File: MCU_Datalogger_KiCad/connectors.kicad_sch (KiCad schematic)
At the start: 4 parts, among them J1 Conn_01x04_Male, J2 Conn_01x04_Male, J3 Conn_01x09_Male, J4 Conn_02x03_Odd_Even

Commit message: Footprint association
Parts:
- J1: footprint (none) -> Connector_PinHeader_2.54mm:PinHeader_1x04_P2.54mm_Vertical
- J2: footprint (none) -> Connector_PinHeader_2.54mm:PinHeader_1x04_P2.54mm_Horizontal
- J3: footprint (none) -> Connector_PinHeader_2.54mm:PinHeader_1x09_P2.54mm_Vertical
- J4: footprint (none) -> Connector_PinHeader_2.54mm:PinHeader_2x03_P2.54mm_Vertical
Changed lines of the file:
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@@
     (property "Reference" "J2" (id 0) (at 65.405 30.48 0))
     (property "Value" "Conn_01x04_Male" (id 1) (at 65.405 33.02 0))
-    (property "Footprint" "" (id 2) (at 64.77 38.1 0)
+    (property "Footprint" "Connector_PinHeader_2.54mm:PinHeader_1x04_P2.54mm_Horizontal" (id 2) (at 64.77 38.1 0)
       (effects (font (size 1.27 1.27)) hide)
     )
@@
     (property "Reference" "J3" (id 0) (at 93.345 25.4 0))
     (property "Value" "Conn_01x09_Male" (id 1) (at 93.345 27.94 0))
-    (property "Footprint" "" (id 2) (at 92.71 40.64 0)
+    (property "Footprint" "Connector_PinHeader_2.54mm:PinHeader_1x09_P2.54mm_Vertical" (id 2) (at 92.71 40.64 0)
       (effects (font (size 1.27 1.27)) hide)
     )
@@
     (property "Reference" "J4" (id 0) (at 118.11 29.21 0))
     (property "Value" "Conn_02x03_Odd_Even" (id 1) (at 118.11 31.75 0))
-    (property "Footprint" "" (id 2) (at 116.84 38.1 0)
+    (property "Footprint" "Connector_PinHeader_2.54mm:PinHeader_2x03_P2.54mm_Vertical" (id 2) (at 116.84 38.1 0)
       (effects (font (size 1.27 1.27)) hide)
     )
@@
     (property "Reference" "J1" (id 0) (at 40.005 31.75 0))
     (property "Value" "Conn_01x04_Male" (id 1) (at 40.005 34.29 0))
-    (property "Footprint" "" (id 2) (at 39.37 39.37 0)
+    (property "Footprint" "Connector_PinHeader_2.54mm:PinHeader_1x04_P2.54mm_Vertical" (id 2) (at 39.37 39.37 0)
       (effects (font (size 1.27 1.27)) hide)
     )

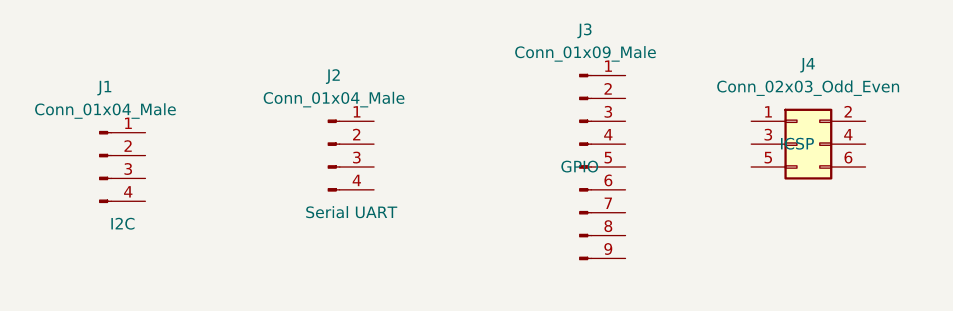
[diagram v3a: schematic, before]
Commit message: Wiring sheet 2
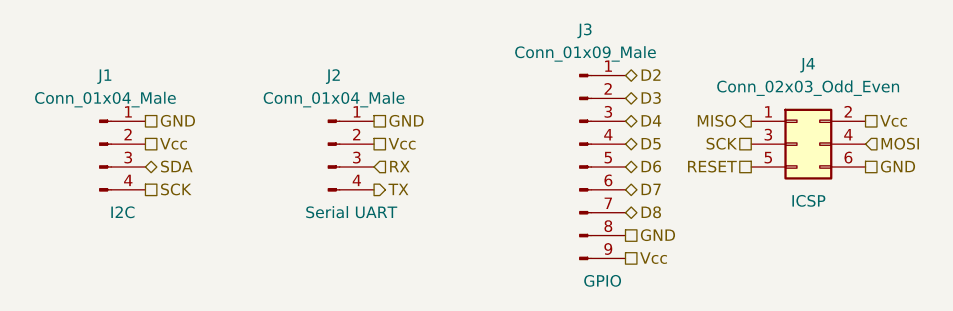
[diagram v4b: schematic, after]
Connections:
- net GND: now reaches J2.1 (Pin_1)
- net GND: now also J1.1 (Pin_1), J3.8 (Pin_8), J4.6 (Pin_6)
- net Vcc: now reaches J2.2 (Pin_2)
- net Vcc: now also J1.2 (Pin_2), J3.9 (Pin_9), J4.2 (Pin_2)
- net RX: now reaches J2.3 (Pin_3)
- net TX: now reaches J2.4 (Pin_4)
- net D2: now reaches J3.1 (Pin_1)
- net D3: now reaches J3.2 (Pin_2)
- net D4: now reaches J3.3 (Pin_3)
- net D5: now reaches J3.4 (Pin_4)
- net D6: now reaches J3.5 (Pin_5)
- net D7: now reaches J3.6 (Pin_6)
- net D8: now reaches J3.7 (Pin_7)
- net MISO: now reaches J4.1 (Pin_1)
- net SCK: now reaches J4.3 (Pin_3)
- net SCK: now also J1.4 (Pin_4)
- net MOSI: now reaches J4.4 (Pin_4)
- net RESET: now reaches J4.5 (Pin_5)
- net SDA: now reaches J1.3 (Pin_3)
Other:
- moved on the sheet: J1
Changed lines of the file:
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@@
 (kicad_sch (version 20211123) (generator eeschema)
   (paper "A4")
+  (hierarchical_label "SCK" (shape passive) (at 44.45 43.18 0)
+    (effects (font (size 1.27 1.27)) (justify left))
+  )
+  (hierarchical_label "D6" (shape bidirectional) (at 97.79 40.64 0)
+    (effects (font (size 1.27 1.27)) (justify left))
+  )
+  (hierarchical_label "RX" (shape input) (at 69.85 40.64 0)
+    (effects (font (size 1.27 1.27)) (justify left))
+  )
+  (hierarchical_label "D7" (shape bidirectional) (at 97.79 43.18 0)
+    (effects (font (size 1.27 1.27)) (justify left))
+  )
+  (hierarchical_label "Vcc" (shape passive) (at 44.45 38.1 0)
+    (effects (font (size 1.27 1.27)) (justify left))
+  )
+  (hierarchical_label "GND" (shape passive) (at 124.46 40.64 0)
+    (effects (font (size 1.27 1.27)) (justify left))
+  )
+  (hierarchical_label "MISO" (shape output) (at 111.76 35.56 180)
+    (effects (font (size 1.27 1.27)) (justify right))
+  )
+  (hierarchical_label "SCK" (shape passive) (at 111.76 38.1 180)
+    (effects (font (size 1.27 1.27)) (justify right))
+  )
+  (hierarchical_label "GND" (shape passive) (at 44.45 35.56 0)
+    (effects (font (size 1.27 1.27)) (justify left))
+  )
+  (hierarchical_label "SDA" (shape bidirectional) (at 44.45 40.64 0)
+    (effects (font (size 1.27 1.27)) (justify left))
+  )
+  (hierarchical_label "D2" (shape bidirectional) (at 97.79 30.48 0)
+    (effects (font (size 1.27 1.27)) (justify left))
+  )
+  (hierarchical_label "D3" (shape bidirectional) (at 97.79 33.02 0)
+    (effects (font (size 1.27 1.27)) (justify left))
+  )
+  (hierarchical_label "D8" (shape bidirectional) (at 97.79 45.72 0)
+    (effects (font (size 1.27 1.27)) (justify left))
+  )
+  (hierarchical_label "Vcc" (shape passive) (at 97.79 50.8 0)
+    (effects (font (size 1.27 1.27)) (justify left))
+  )
+  (hierarchical_label "TX" (shape output) (at 69.85 43.18 0)
+    (effects (font (size 1.27 1.27)) (justify left))
+  )
+  (hierarchical_label "GND" (shape passive) (at 97.79 48.26 0)
+    (effects (font (size 1.27 1.27)) (justify left))
+  )
+  (hierarchical_label "RESET" (shape passive) (at 111.76 40.64 180)
+    (effects (font (size 1.27 1.27)) (justify right))
+  )
+  (hierarchical_label "D5" (shape bidirectional) (at 97.79 38.1 0)
+    (effects (font (size 1.27 1.27)) (justify left))
+  )
+  (hierarchical_label "Vcc" (shape passive) (at 69.85 38.1 0)
+    (effects (font (size 1.27 1.27)) (justify left))
+  )
+  (hierarchical_label "Vcc" (shape passive) (at 124.46 35.56 0)
+    (effects (font (size 1.27 1.27)) (justify left))
+  )
+  (hierarchical_label "MOSI" (shape input) (at 124.46 38.1 0)
+    (effects (font (size 1.27 1.27)) (justify left))
+  )
+  (hierarchical_label "D4" (shape bidirectional) (at 97.79 35.56 0)
+    (effects (font (size 1.27 1.27)) (justify left))
+  )
+  (hierarchical_label "GND" (shape passive) (at 69.85 35.56 0)
+    (effects (font (size 1.27 1.27)) (justify left))
+  )
   (symbol (lib_id "Connector:Conn_01x04_Male") (at 64.77 38.1 0) (unit 1)
     (in_bom yes) (on_board yes)
@@
   )
   (symbol (lib_id "Connector:Conn_01x09_Male") (at 92.71 40.64 0) (unit 1)
-    (in_bom yes) (on_board yes) (fields_autoplaced)
+    (in_bom yes) (on_board yes)
     (property "Reference" "J3" (id 0) (at 93.345 25.4 0))
     (property "Value" "Conn_01x09_Male" (id 1) (at 93.345 27.94 0))
@@
       (effects (font (size 1.27 1.27)) hide)
     )
-    (property "Purpose" "GPIO" (id 4) (at 92.71 40.64 0))
+    (property "Purpose" "GPIO" (id 4) (at 95.25 53.34 0))
     (pin "1")
     (pin "2")
@@
   )
   (symbol (lib_id "Connector_Generic:Conn_02x03_Odd_Even") (at 116.84 38.1 0) (unit 1)
-    (in_bom yes) (on_board yes) (fields_autoplaced)
+    (in_bom yes) (on_board yes)
     (property "Reference" "J4" (id 0) (at 118.11 29.21 0))
     (property "Value" "Conn_02x03_Odd_Even" (id 1) (at 118.11 31.75 0))
@@
       (effects (font (size 1.27 1.27)) hide)
     )
-    (property "Purpose" "ICSP" (id 4) (at 116.84 38.1 0))
+    (property "Purpose" "ICSP" (id 4) (at 118.11 44.45 0))
     (pin "1")
     (pin "2")
@@
     (pin "6")
   )
-  (symbol (lib_id "Connector:Conn_01x04_Male") (at 39.37 39.37 0) (unit 1)
+  (symbol (lib_id "Connector:Conn_01x04_Male") (at 39.37 38.1 0) (unit 1)
     (in_bom yes) (on_board yes)
-    (property "Reference" "J1" (id 0) (at 40.005 31.75 0))
-    (property "Value" "Conn_01x04_Male" (id 1) (at 40.005 34.29 0))
-    (property "Footprint" "Connector_PinHeader_2.54mm:PinHeader_1x04_P2.54mm_Vertical" (id 2) (at 39.37 39.37 0)
+    (property "Reference" "J1" (id 0) (at 40.005 30.48 0))
+    (property "Value" "Conn_01x04_Male" (id 1) (at 40.005 33.02 0))
+    (property "Footprint" "Connector_PinHeader_2.54mm:PinHeader_1x04_P2.54mm_Vertical" (id 2) (at 39.37 38.1 0)
       (effects (font (size 1.27 1.27)) hide)
     )
-    (property "Datasheet" "~" (id 3) (at 39.37 39.37 0)
+    (property "Datasheet" "~" (id 3) (at 39.37 38.1 0)
       (effects (font (size 1.27 1.27)) hide)
     )
-    (property "Purpose" "I2C" (id 4) (at 41.91 46.99 0))
+    (property "Purpose" "I2C" (id 4) (at 41.91 45.72 0))
     (pin "1")
     (pin "2")
